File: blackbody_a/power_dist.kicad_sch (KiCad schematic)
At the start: 31 parts, among them IC1 LM76202QPWPRQ1, U4 TPS5403DR

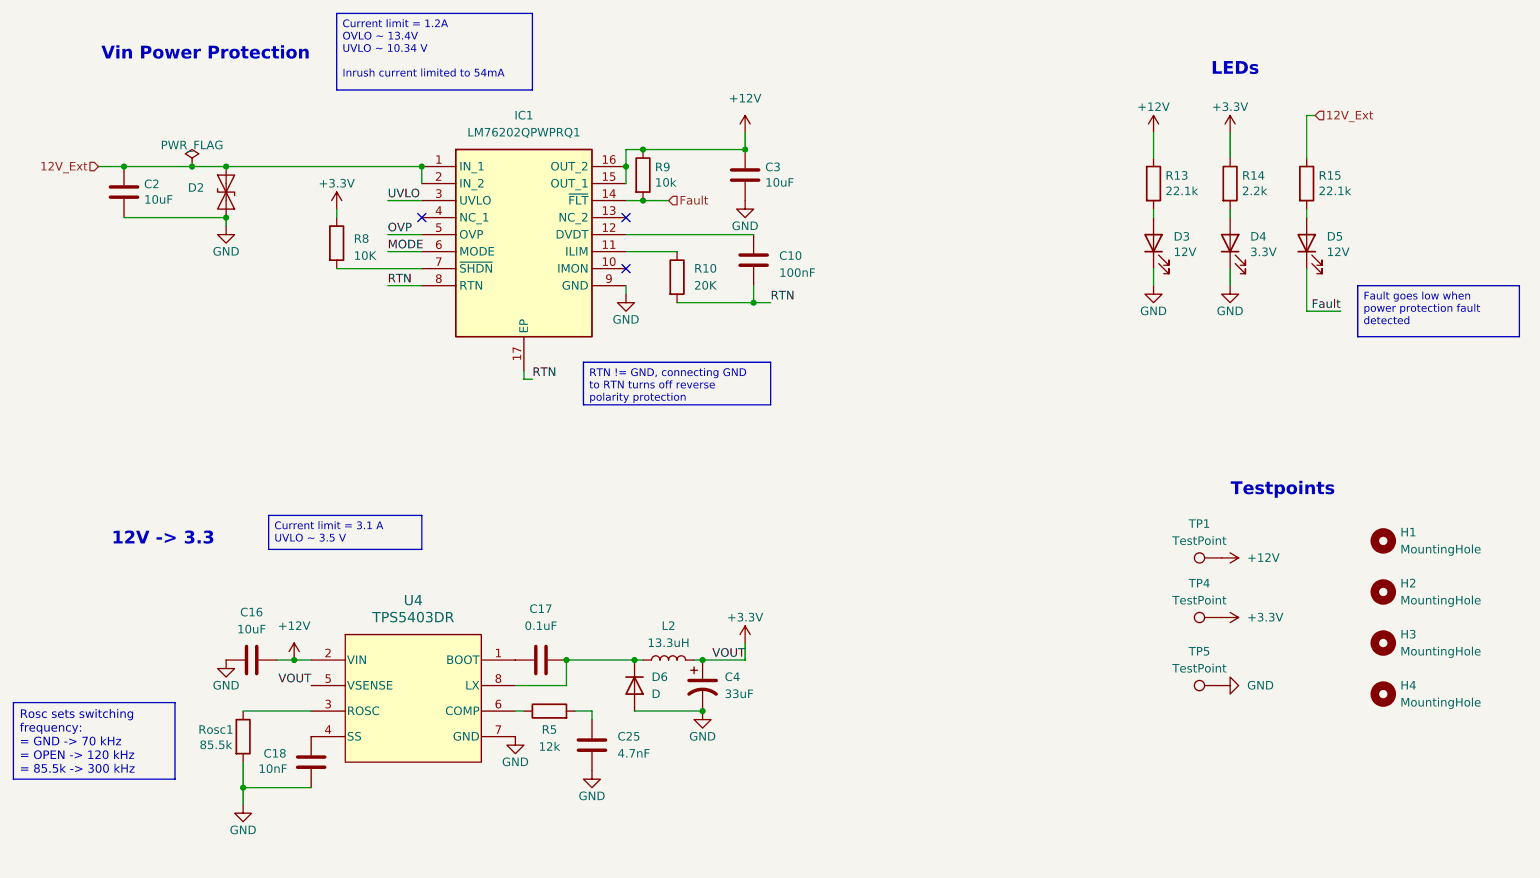
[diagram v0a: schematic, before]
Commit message: layout updates
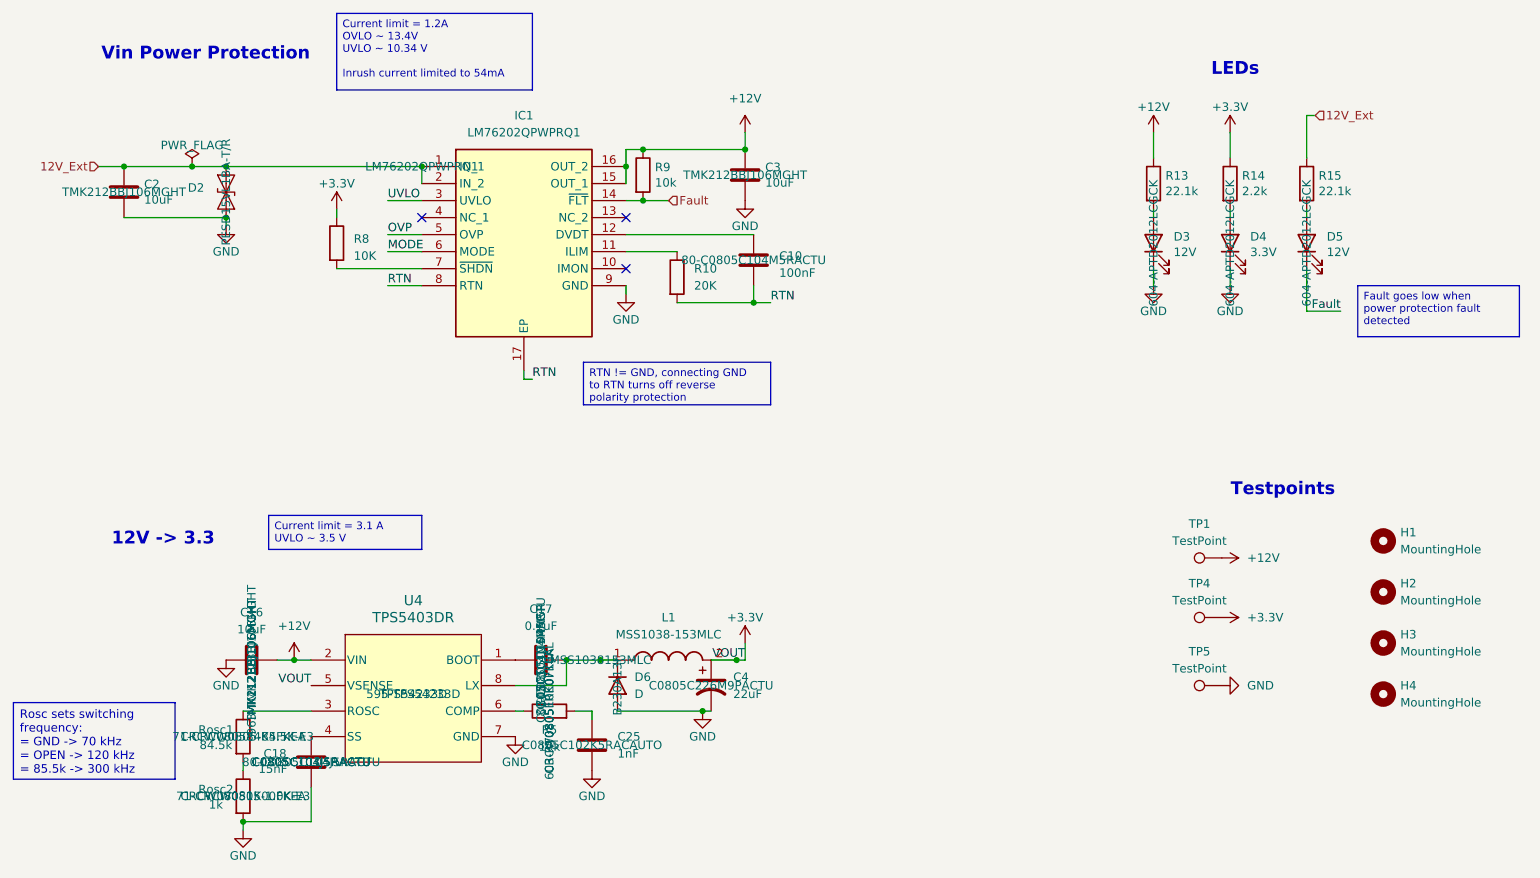
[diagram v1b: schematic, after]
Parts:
- removed L2: 13.3uH, Inductor_SMD:L_0805_2012Metric, symbol Device:L
- added L1: MSS1038-153MLC, blackbody_a:INDPM102100X400N, symbol MSS1038-153MLC:MSS1038-153MLC
- added Rosc2: 1k, Resistor_SMD:R_0805_2012Metric, symbol Device:R
- C10: Manufacturer_Part_Number (none) -> 80-C0805C104M5RACTU; Mouser Part Number 80-C0805C104M5R -> 80-C0805C104M5RACTU; PN (none) -> C0805C104M5RACTU
- C16: Manufacturer_Part_Number (none) -> TMK212BBJ106MGHT; Mouser Part Number (none) -> 963-TMK212BBJ106MGHT; PN (none) -> TMK212BBJ106MGHT
- C17: Manufacturer_Part_Number (none) -> C0805C104M5R; Mouser Part Number (none) -> 80-C0805C104M5R; PN (none) -> C0805C104M5RACTU
- C18: value 10nF -> 15nF; Manufacturer_Part_Number (none) -> C0805C104J5RACTU; Mouser Part Number (none) -> 80-C0805C104J5RACTU; PN (none) -> C0805C103J5RACTU
- C2, C3: Manufacturer_Part_Number (none) -> TMK212BBJ106MGHT; Mouser Part Number 581-22201C106KAT2A -> 963-TMK212BBJ106MGHT; PN (none) -> TMK212BBJ106MGHT
- C25: value 4.7nF -> 1nF; PN (none) -> C0805C102K5RACAUTO
- C4: value 33uF -> 22uF; PN (none) -> C0805C226M9PACTU
- D2: Manufacturer_Part_Number (none) -> PESD15VL1BA-T/R; Mouser Part Number 771-PESD15VL1BA-T/R -> 821-BZT52C12S; PN (none) -> BZT52C12S
- D3, D4, D5: Manufacturer_Part_Number (none) -> 604-APTD2012LCGCK; PN (none) -> APTD2012LCGCK
- D6: footprint Diode_SMD:D_0805_2012Metric -> blackbodies:SMA_DIO; PN (none) -> B230A13F
- IC1: PN (none) -> LM76202QPWPRQ1
- R10, R13, R15: PN (none) -> CRCW080520K0FKEA
- R14: Mouser Part Number Inventory -> 71-CRCW0805-2.2K-E3; PN (none) -> CRCW08052K20FKEA
- R5: value 12k -> 10k; Mouser Part Number (none) -> 603-RT0805FRE0710KL; PN (none) -> CRCW080510K0FKEA
- R8: PN (none) -> RT0805FRE0710KL
- R9: Mouser Part Number 71-CRCW0805100KFKEAC -> 603-RT0805FRE0710KL; PN (none) -> CRCW080510K0FKEA
- Rosc1: value 85.5k -> 84.5k; Mouser Part Number (none) -> 71-CRCW0805-84.5K-E3; PN (none) -> CRCW080584K5FKEA
- U4: Mouser Part Number (none) -> 595-TPS54233D; PN (none) -> TPS54233D
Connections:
- net +3.3V: now also L1.2
- net GND: now also Rosc2.2; no longer Rosc1.2
- net at C17.2, D6.1 (K), U4.8 (LX): now also L1.1
- new net: Rosc1.2, Rosc2.1
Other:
- moved on the sheet: C4, D6
